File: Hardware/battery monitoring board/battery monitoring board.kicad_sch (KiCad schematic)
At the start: 3 parts, among them J7 Conn_01x02, J8 Conn_01x02

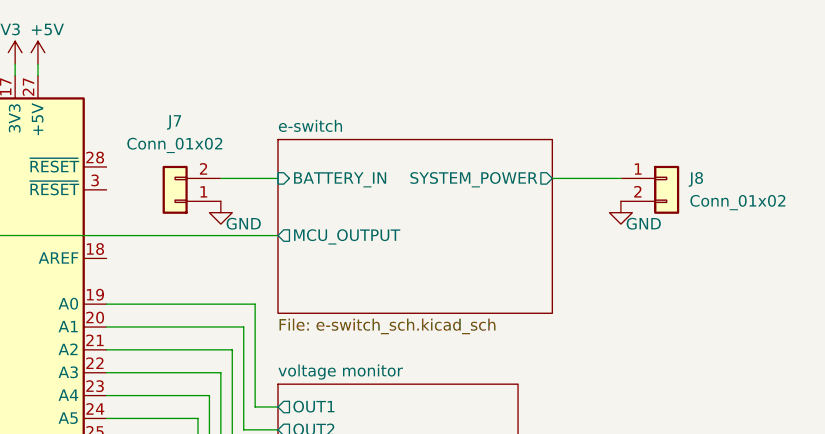
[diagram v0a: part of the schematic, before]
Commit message: Updated reference labels
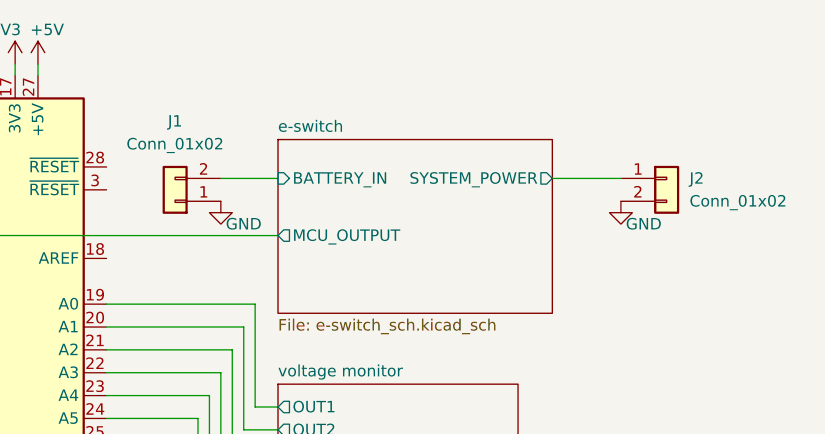
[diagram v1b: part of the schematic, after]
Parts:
- renumbered J7 to J1, J8 to J2
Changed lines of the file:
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@@
   (symbol (lib_id "Connector_Generic:Conn_01x02") (at 196.85 71.12 0) (unit 1)
     (in_bom yes) (on_board yes) (dnp no) (fields_autoplaced)
-    (property "Reference" "J8" (at 199.39 71.12 0)
+    (property "Reference" "J2" (at 199.39 71.12 0)
       (effects (font (size 1.27 1.27)) (justify left))
     )
@@
       (project "battery monitoring board"
         (path "/bf623d80-ca5a-491f-9daa-4dffbeba5279"
-          (reference "J8") (unit 1)
+          (reference "J2") (unit 1)
         )
       )
@@
   (symbol (lib_id "power:+3V3") (at 124.46 58.42 0) (unit 1)
     (in_bom yes) (on_board yes) (dnp no)
-    (property "Reference" "#PWR019" (at 124.46 62.23 0)
+    (property "Reference" "#PWR02" (at 124.46 62.23 0)
       (effects (font (size 1.27 1.27)) hide)
     )
@@
       (project "battery monitoring board"
         (path "/bf623d80-ca5a-491f-9daa-4dffbeba5279"
-          (reference "#PWR019") (unit 1)
+          (reference "#PWR02") (unit 1)
         )
       )
@@
   (symbol (lib_id "PCM_4ms_Power-symbol:GND") (at 191.77 73.66 0) (unit 1)
     (in_bom yes) (on_board yes) (dnp no)
-    (property "Reference" "#PWR020" (at 191.77 80.01 0)
+    (property "Reference" "#PWR05" (at 191.77 80.01 0)
       (effects (font (size 1.27 1.27)) hide)
     )
@@
       (project "battery monitoring board"
         (path "/bf623d80-ca5a-491f-9daa-4dffbeba5279"
-          (reference "#PWR020") (unit 1)
+          (reference "#PWR05") (unit 1)
         )
       )
@@
   (symbol (lib_id "Connector_Generic:Conn_01x02") (at 142.24 73.66 180) (unit 1)
     (in_bom yes) (on_board yes) (dnp no) (fields_autoplaced)
-    (property "Reference" "J7" (at 142.24 64.77 0)
+    (property "Reference" "J1" (at 142.24 64.77 0)
       (effects (font (size 1.27 1.27)))
     )
@@
       (project "battery monitoring board"
         (path "/bf623d80-ca5a-491f-9daa-4dffbeba5279"
-          (reference "J7") (unit 1)
+          (reference "J1") (unit 1)
         )
       )
@@
   (symbol (lib_id "PCM_4ms_Power-symbol:+5V") (at 127 58.42 0) (unit 1)
     (in_bom yes) (on_board yes) (dnp no)
-    (property "Reference" "#PWR02" (at 127 62.23 0)
+    (property "Reference" "#PWR03" (at 127 62.23 0)
       (effects (font (size 1.27 1.27)) hide)
     )
@@
       (project "battery monitoring board"
         (path "/bf623d80-ca5a-491f-9daa-4dffbeba5279"
-          (reference "#PWR02") (unit 1)
+          (reference "#PWR03") (unit 1)
         )
       )
@@
   (symbol (lib_id "PCM_4ms_Power-symbol:GND") (at 147.32 73.66 0) (unit 1)
     (in_bom yes) (on_board yes) (dnp no)
-    (property "Reference" "#PWR021" (at 147.32 80.01 0)
+    (property "Reference" "#PWR04" (at 147.32 80.01 0)
       (effects (font (size 1.27 1.27)) hide)
     )
@@
       (project "battery monitoring board"
         (path "/bf623d80-ca5a-491f-9daa-4dffbeba5279"
-          (reference "#PWR021") (unit 1)
+          (reference "#PWR04") (unit 1)
         )
       )

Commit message: Revert "Updated reference labels"
This reverts commit 7ccd23260c988ead49c0bcfa936e50f6d09a7000.
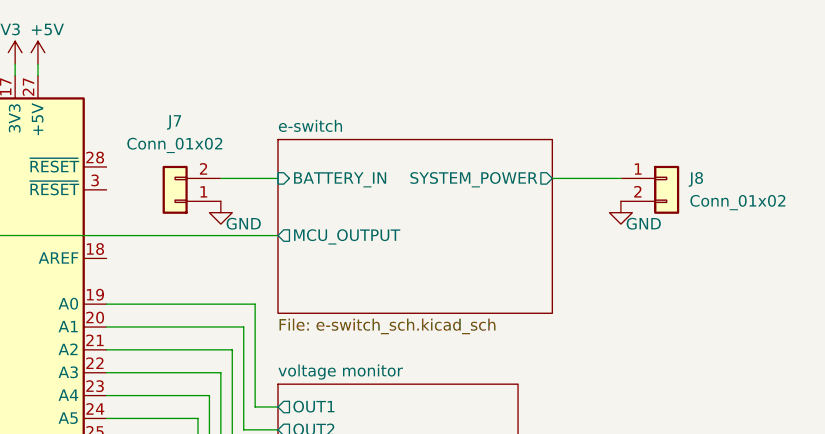
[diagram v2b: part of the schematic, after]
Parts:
- renumbered J1 to J7, J2 to J8
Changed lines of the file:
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@@
   (symbol (lib_id "Connector_Generic:Conn_01x02") (at 196.85 71.12 0) (unit 1)
     (in_bom yes) (on_board yes) (dnp no) (fields_autoplaced)
-    (property "Reference" "J2" (at 199.39 71.12 0)
+    (property "Reference" "J8" (at 199.39 71.12 0)
       (effects (font (size 1.27 1.27)) (justify left))
     )
@@
       (project "battery monitoring board"
         (path "/bf623d80-ca5a-491f-9daa-4dffbeba5279"
-          (reference "J2") (unit 1)
+          (reference "J8") (unit 1)
         )
       )
@@
   (symbol (lib_id "power:+3V3") (at 124.46 58.42 0) (unit 1)
     (in_bom yes) (on_board yes) (dnp no)
-    (property "Reference" "#PWR02" (at 124.46 62.23 0)
+    (property "Reference" "#PWR019" (at 124.46 62.23 0)
       (effects (font (size 1.27 1.27)) hide)
     )
@@
       (project "battery monitoring board"
         (path "/bf623d80-ca5a-491f-9daa-4dffbeba5279"
-          (reference "#PWR02") (unit 1)
+          (reference "#PWR019") (unit 1)
         )
       )
@@
   (symbol (lib_id "PCM_4ms_Power-symbol:GND") (at 191.77 73.66 0) (unit 1)
     (in_bom yes) (on_board yes) (dnp no)
-    (property "Reference" "#PWR05" (at 191.77 80.01 0)
+    (property "Reference" "#PWR020" (at 191.77 80.01 0)
       (effects (font (size 1.27 1.27)) hide)
     )
@@
       (project "battery monitoring board"
         (path "/bf623d80-ca5a-491f-9daa-4dffbeba5279"
-          (reference "#PWR05") (unit 1)
+          (reference "#PWR020") (unit 1)
         )
       )
@@
   (symbol (lib_id "Connector_Generic:Conn_01x02") (at 142.24 73.66 180) (unit 1)
     (in_bom yes) (on_board yes) (dnp no) (fields_autoplaced)
-    (property "Reference" "J1" (at 142.24 64.77 0)
+    (property "Reference" "J7" (at 142.24 64.77 0)
       (effects (font (size 1.27 1.27)))
     )
@@
       (project "battery monitoring board"
         (path "/bf623d80-ca5a-491f-9daa-4dffbeba5279"
-          (reference "J1") (unit 1)
+          (reference "J7") (unit 1)
         )
       )
@@
   (symbol (lib_id "PCM_4ms_Power-symbol:+5V") (at 127 58.42 0) (unit 1)
     (in_bom yes) (on_board yes) (dnp no)
-    (property "Reference" "#PWR03" (at 127 62.23 0)
+    (property "Reference" "#PWR02" (at 127 62.23 0)
       (effects (font (size 1.27 1.27)) hide)
     )
@@
       (project "battery monitoring board"
         (path "/bf623d80-ca5a-491f-9daa-4dffbeba5279"
-          (reference "#PWR03") (unit 1)
+          (reference "#PWR02") (unit 1)
         )
       )
@@
   (symbol (lib_id "PCM_4ms_Power-symbol:GND") (at 147.32 73.66 0) (unit 1)
     (in_bom yes) (on_board yes) (dnp no)
-    (property "Reference" "#PWR04" (at 147.32 80.01 0)
+    (property "Reference" "#PWR021" (at 147.32 80.01 0)
       (effects (font (size 1.27 1.27)) hide)
     )
@@
       (project "battery monitoring board"
         (path "/bf623d80-ca5a-491f-9daa-4dffbeba5279"
-          (reference "#PWR04") (unit 1)
+          (reference "#PWR021") (unit 1)
         )
       )
